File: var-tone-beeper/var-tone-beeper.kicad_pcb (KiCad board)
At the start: 2 copper layers, 194.9 x 118.7 mm, 11 parts, among them SW1 SW_Push, U1 NE555P

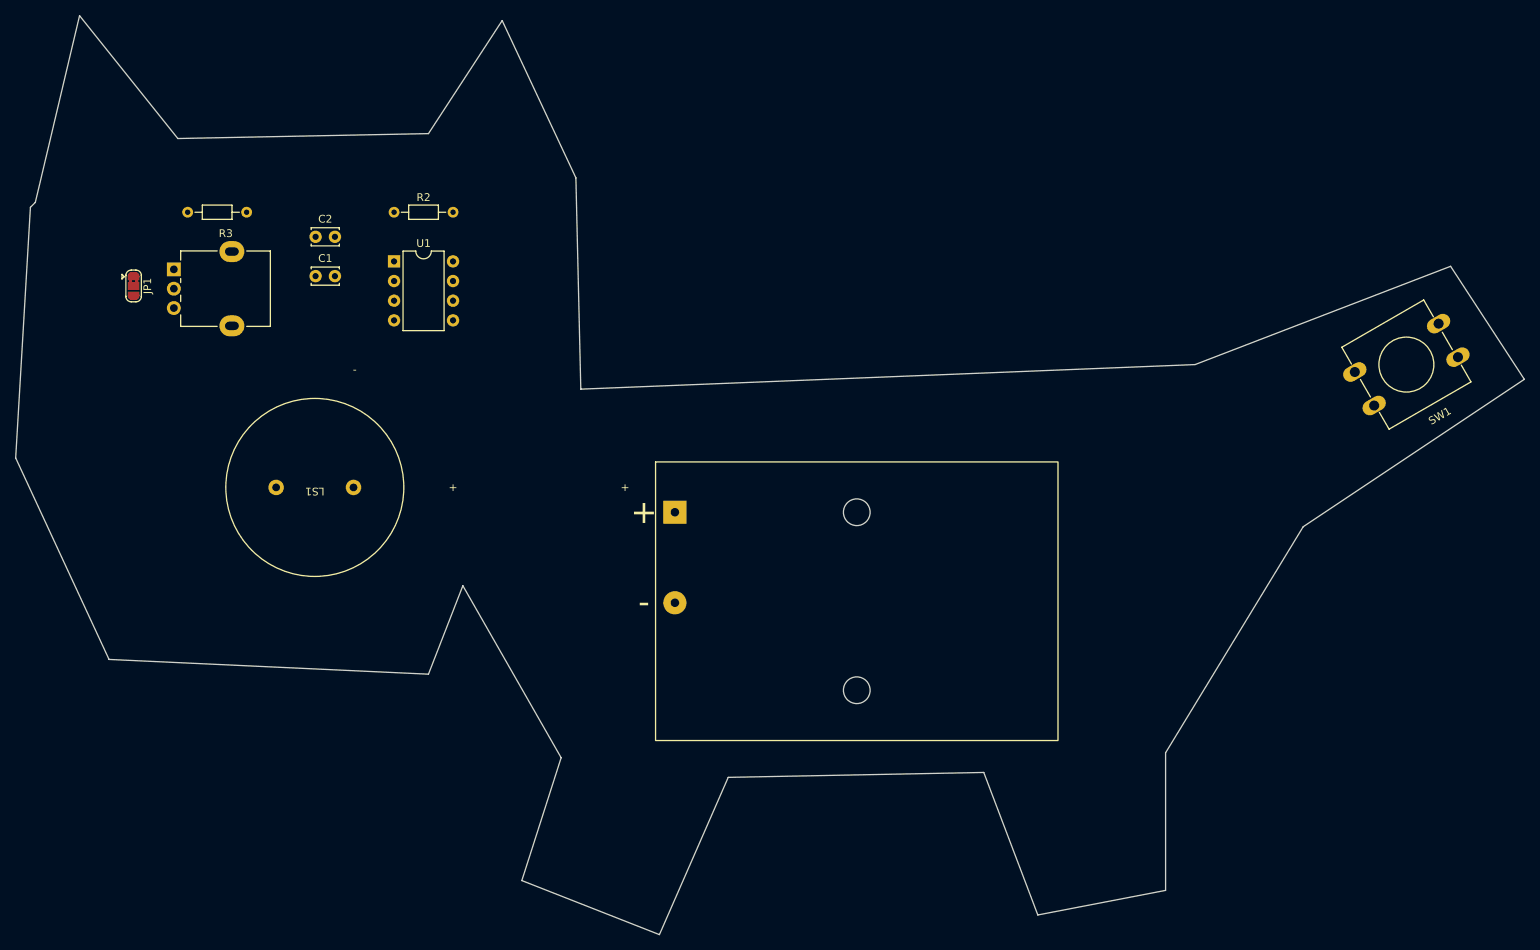
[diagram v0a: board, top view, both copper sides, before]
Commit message: ver-tone-beeper: v1 ordered
Reduced board size
Ordered

JLCPCB cost: 10x for $14.10 + $8.36 shipping/tax
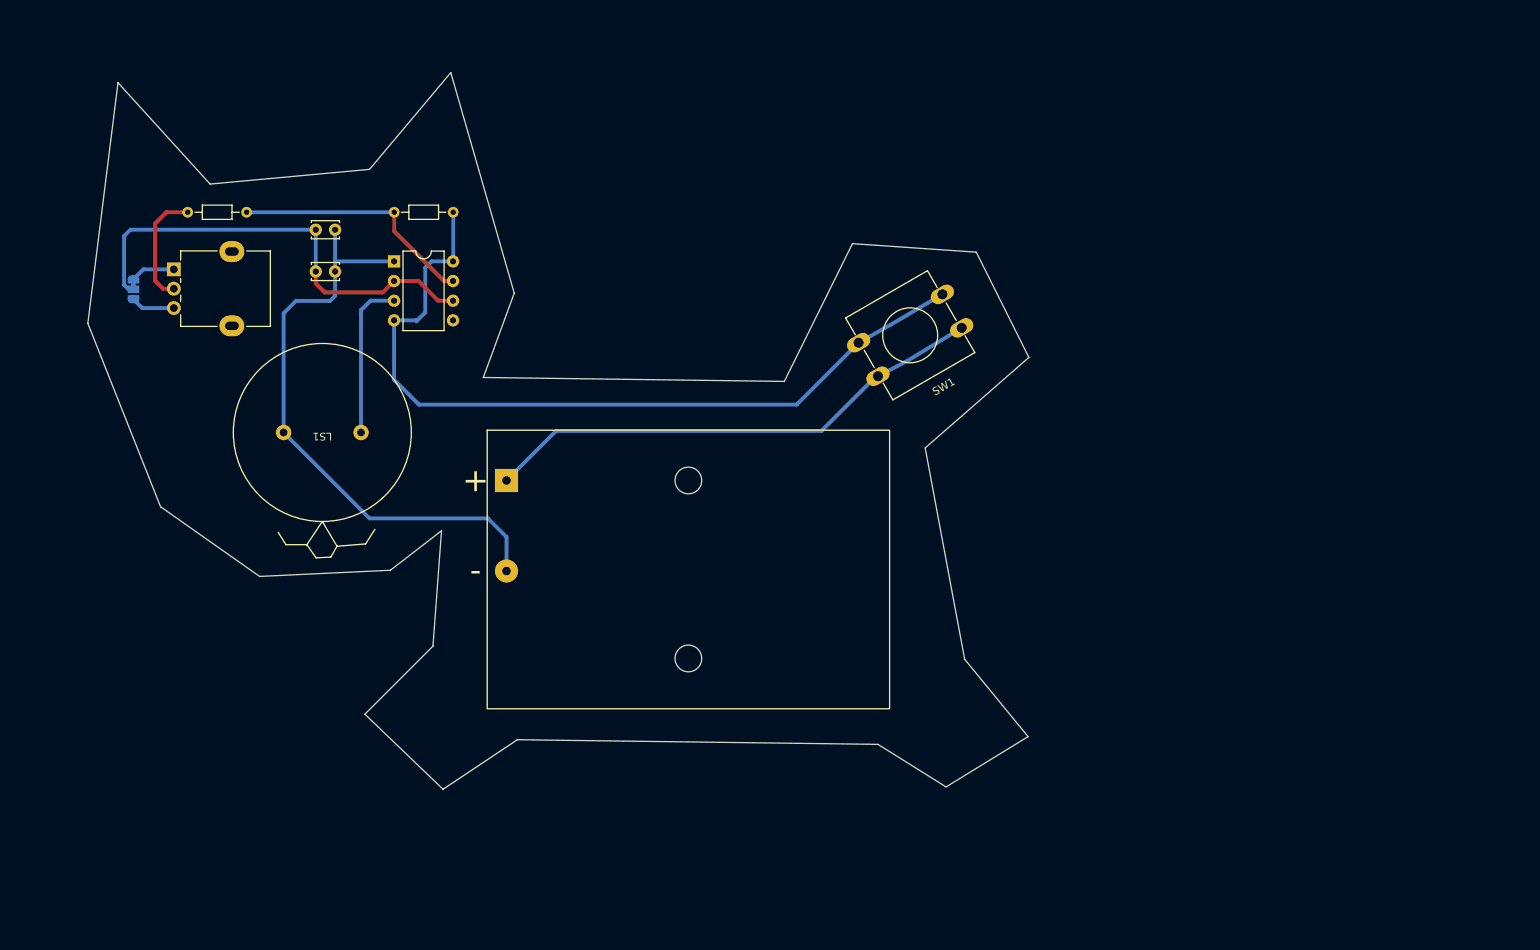
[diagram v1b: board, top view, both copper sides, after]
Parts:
- JP1: footprint Jumper:SolderJumper-3_P1.3mm_Bridged2Bar12_RoundedPad1.0x1.5mm -> Jumper:SolderJumper-3_P1.3mm_Bridged12_RoundedPad1.0x1.5mm; moved to B.Cu
- moved SW1 64.2 mm to (201.6, 81.0)
- moved G*** 59.6 mm to (180.9, 119.6)
- moved BT1 22.1 mm to (140.3, 94.2)
- moved R2 7.64 mm to (135.9, 66.0), turned to 180 degrees
- moved LS1 7.17 mm to (119.0, 94.5)
- moved C2 0.92 mm to (118.2, 68.3)
- moved C1 0.60 mm to (118.2, 73.7)
- moved JP1 0.44 mm to (94.6, 76.0)
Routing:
- net Net-(U1-R): track 0.00 -> 105.5 mm
- net Net-(BT1--): track 0.00 -> 77.9 mm
- net Net-(BT1-+): track 0.00 -> 66.1 mm
- net Net-(JP1-C): track 0.00 -> 59.7 mm
- net Net-(U1-DIS): track 0.00 -> 31.8 mm
- net Net-(U1-Q): track 0.00 -> 20.4 mm
- net Net-(R1-Pad2): track 0.00 -> 15.0 mm
- net Net-(JP1-A): track 0.00 -> 5.75 mm
- net Net-(JP1-B): track 0.00 -> 5.68 mm
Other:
- board size 194.9 x 118.7 mm -> 121.6 x 92.6 mm
- board text removed: "+"
- board text removed: "-"
